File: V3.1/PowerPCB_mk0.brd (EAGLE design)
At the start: 171.9 x 151.6 mm, 124 parts, among them CON1 PINHEAD_1X12-2.54-FEMALE, CON2 PINHEAD_1X06-2.54-FEMALE, CON3 PINHEAD_1X02-2.54-FEMALE, CON4 PINHEAD_1X06-2.54-FEMALE, CON7 PINHEAD_1X06-2.54-FEMALE, IC1 TPS54560B, IC10 TPS54260, IC2 TPS54560B, IC3 TPS54560B, IC4 TPS54560B, IC5 INA169, J1 CONNECTION-7MM, M1 BATTERY_CON-XT30-RA, M2 BATTERY_CON-XT30-RA, M3 BATTERY_CON-XT30-RA, M4 BATTERY_CON-XT30-RA, M5 BATTERY_CON-XT30-RA, M6 BATTERY_CON-XT30-RA, M7 BATTERY_CON-XT30-RA, Q1 IRFR2407PBF, Q2 IRFR2407PBF, Q3 IRFR2407PBF

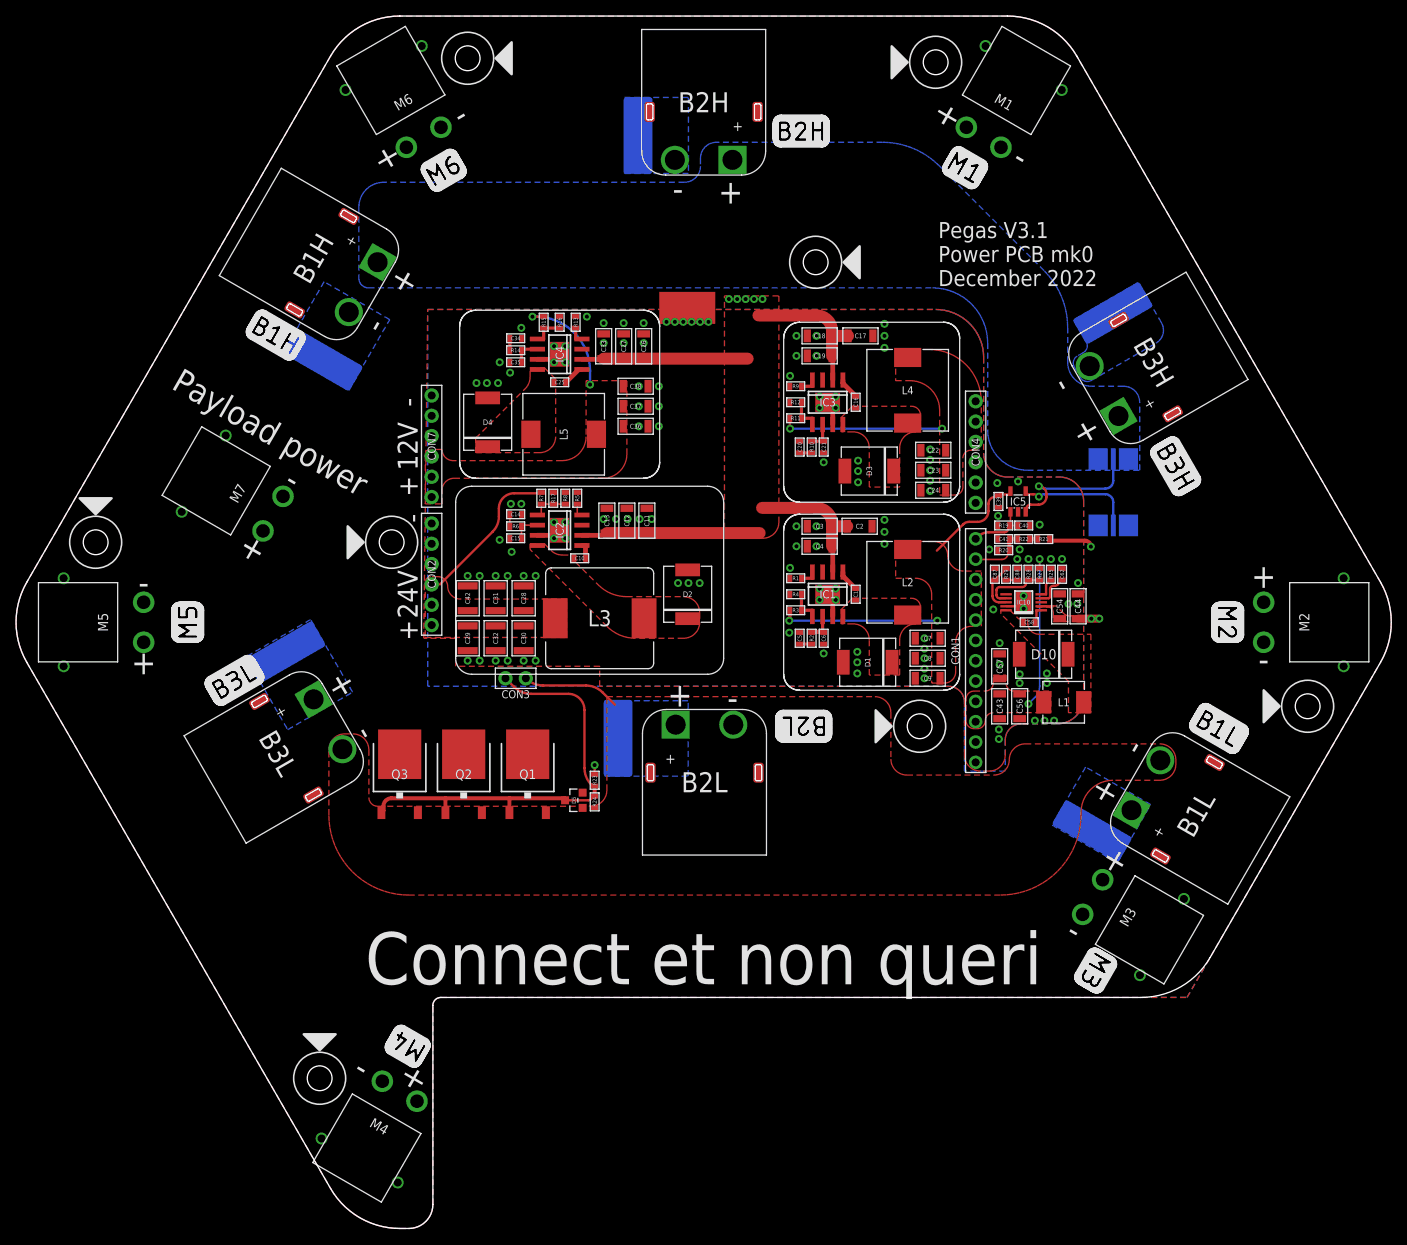
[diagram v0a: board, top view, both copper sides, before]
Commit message: silk updates
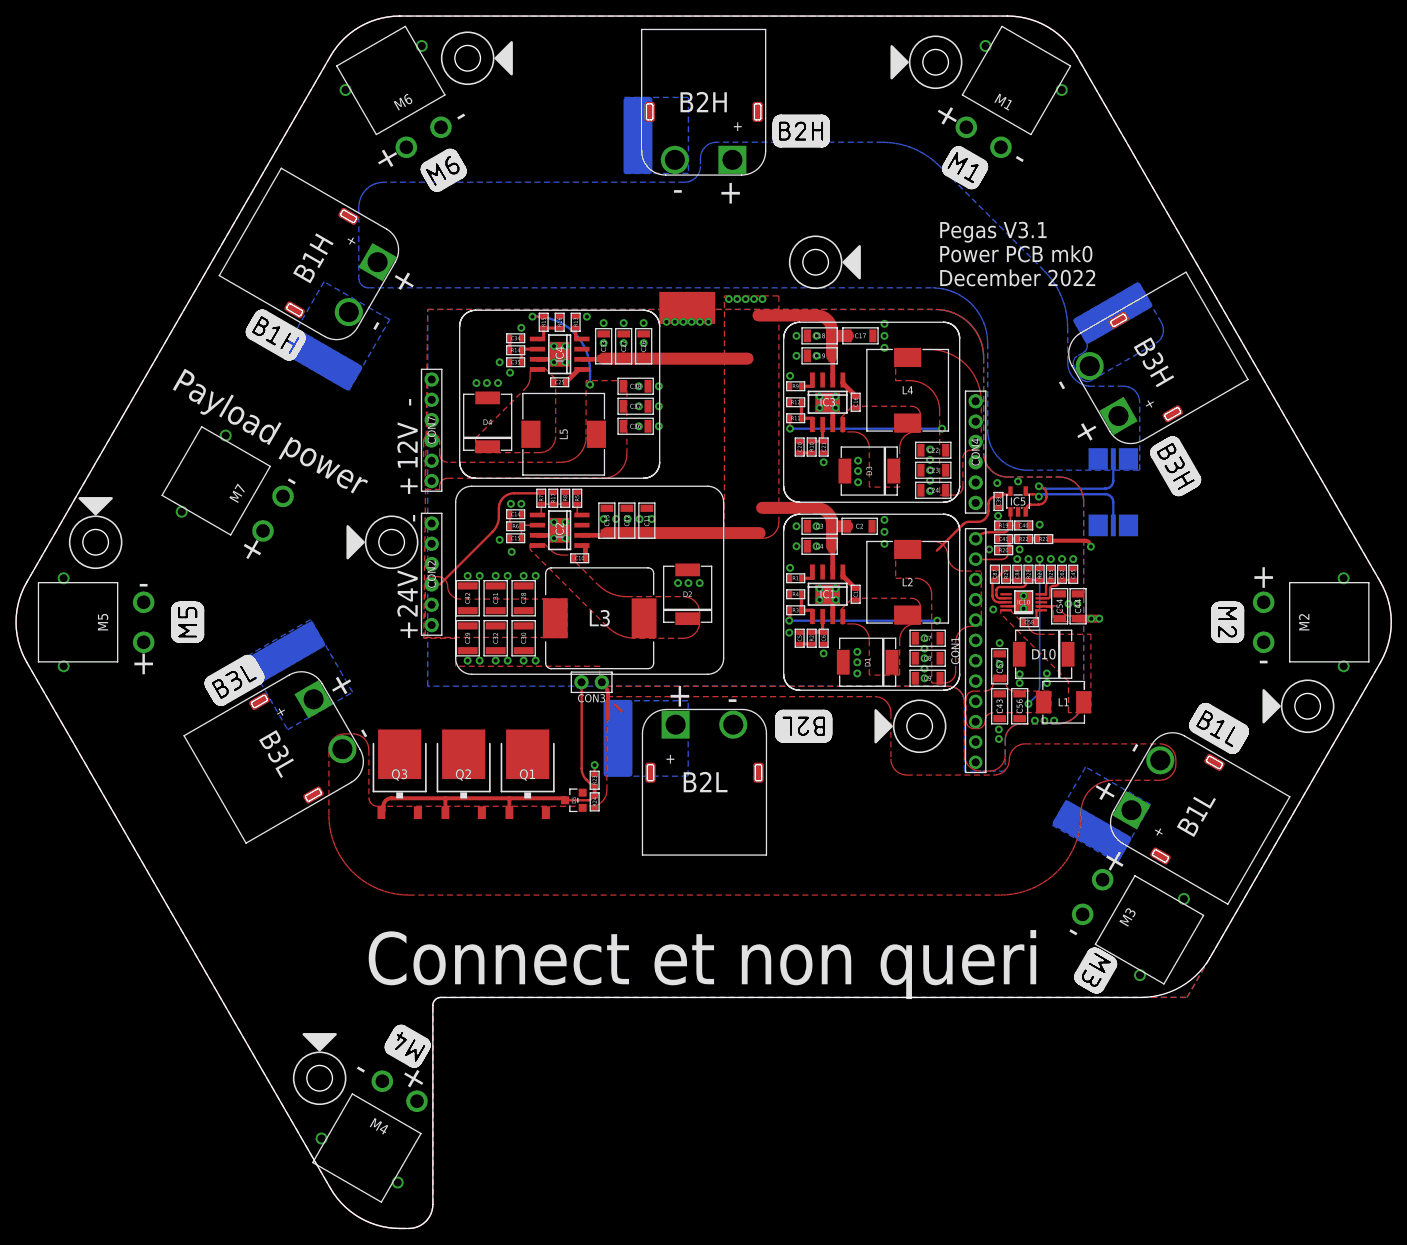
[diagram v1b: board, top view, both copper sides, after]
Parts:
- added C45: 4700p, rc:C0603
- C39: value 0.1uF -> 0.1u
- C62: value 10n -> 4700p
- R20, R23: value 10K2 -> 10K
- moved CON3 9.51 mm to (-14.0, -7.50)
- moved CON7 2.00 mm to (-34.0, 24.0)
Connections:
- net GND: now also C45.2
- net N$20: now also C45.1
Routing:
- net PWRSW: track 54.4 -> 46.7 mm
- net BATNEG: track 12.1 -> 5.94 mm
- net N$20: track 4.07 -> 5.47 mm

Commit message: Minor fixes here and there
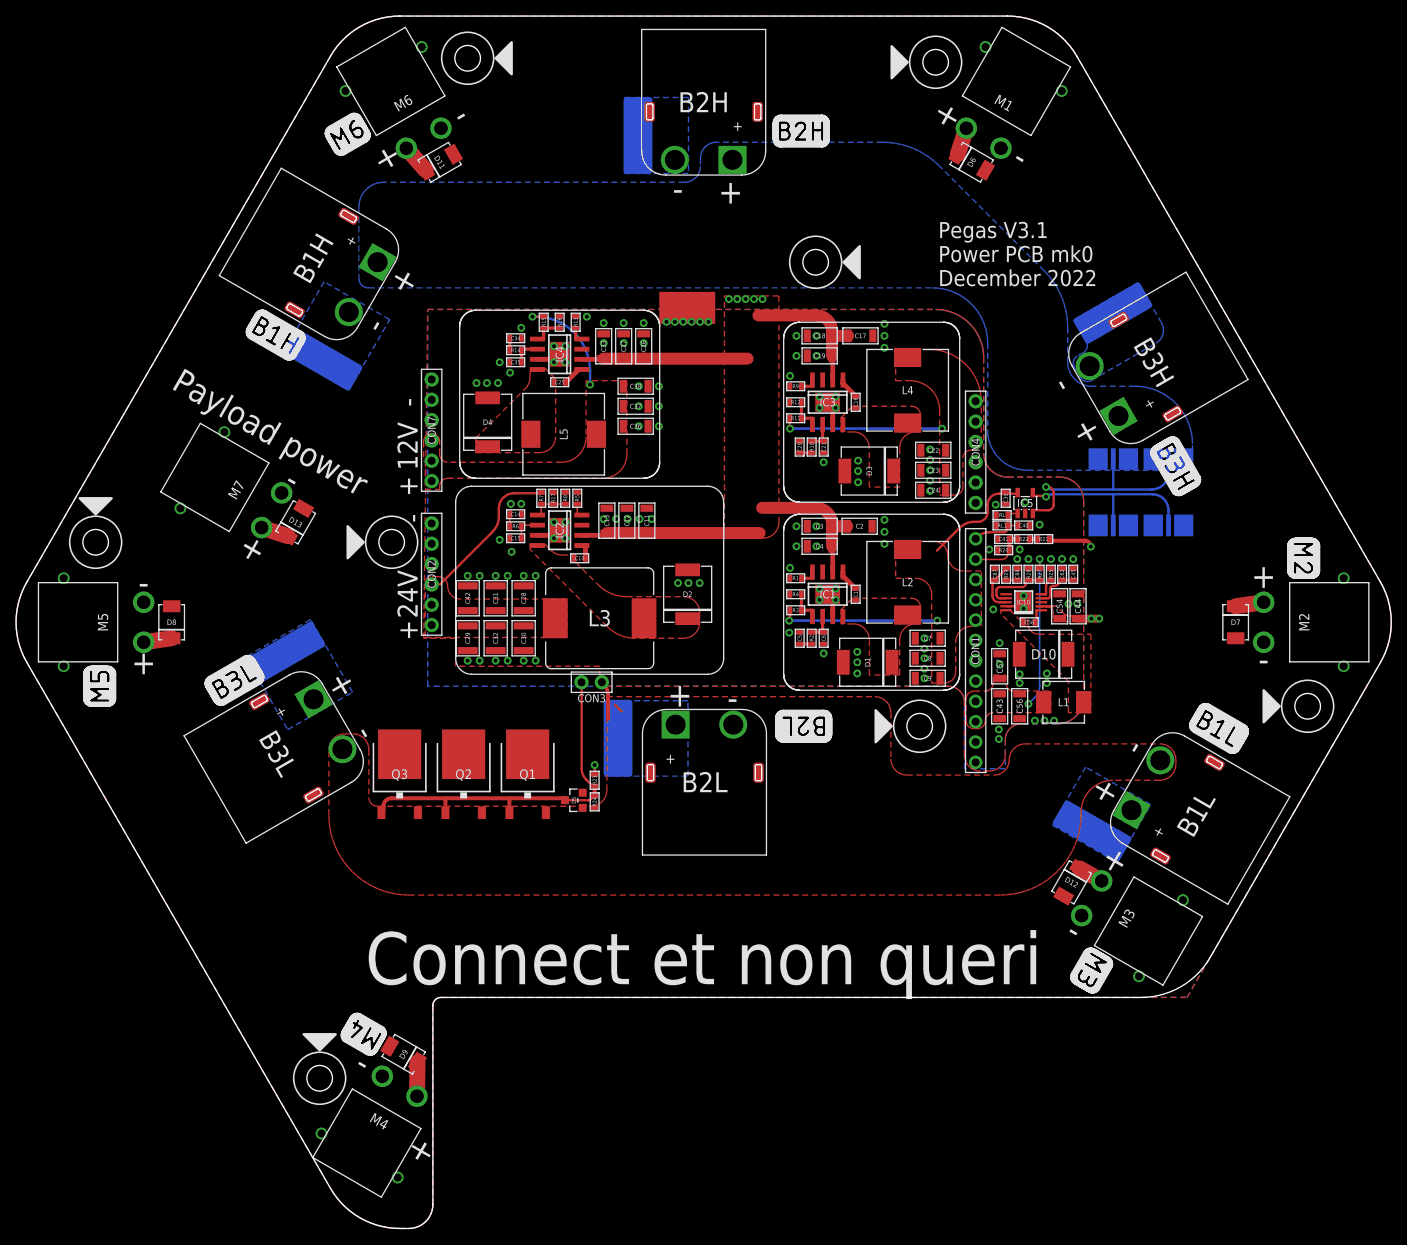
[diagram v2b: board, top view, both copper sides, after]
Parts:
- removed R19: 82K, rc:R0603
- added D11, D12, D13, D6, D7, D8, D9: SMBJ51CA-SMB, TVS_diodes:DO-214AA(SMB)
- added R26: 700 µOhms, SHUNT_RESISTORS:R3920-KELVIN
- added RL: 53K6, rc:R0603
- added RL1: DNM, rc:R0603
- R18: value 200 µOhms -> 700 µOhms
- R21: value 82K -> 143K
- R22: value 82K -> 18K
- moved C39 0.98 mm to (37.8, 15.5)
- moved IC5 0.92 mm to (40.2, 14.9)
- moved M4 0.62 mm to (-38.0, -58.0)
- moved M7 0.46 mm to (-54.0, 14.0)
- moved M3 0.20 mm to (48.5, -34.5)
- moved M6 0.12 mm to (-35.0, 60.5)
- moved M1 0.12 mm to (35.0, 60.5)
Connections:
- net BATT_CURRENT: now also RL.2, RL1.2; no longer R19.2
- net GND: now also RL.1, RL1.1; no longer R19.1
- net N$19: now also R26.S2
- net N$21: now also R26.S1
- net PGND: now also D11.A, D12.A, D13.A, D6.A, D7.A, D8.A, D9.A
- net VBAT: now also D11.C, D12.C, D13.C, D6.C, D7.C, D8.C, D9.C, R26.2, R26.22
- net VDC: now also R26.1, R26.11
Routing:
- net VBAT: track 90.9 -> 115.9 mm
- net N$21: track 17.7 -> 27.8 mm
- net N$19: track 14.8 -> 24.1 mm
- net BATT_CURRENT: track 7.78 -> 8.68 mm
- net 5VFMU: track 32.9 -> 33.6 mm
- net GND: vias 127 -> 126
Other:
- board text added: "25 mm"
- board text added: "Apply heatsink here if needed"
- board text added: "Use 11 mm M3 male to female PCB standoffs between the PCBs"
